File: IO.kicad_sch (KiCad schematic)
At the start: 9 parts, among them J10 Conn_01x04_Pin, J2 Conn_01x02_Pin, J3 Conn_01x02_Pin, J4 Conn_01x02_Pin, J5 Conn_01x02_Pin, J6 Conn_01x02_Pin, J7 Conn_01x04_Pin, J8 Conn_01x04_Pin, J9 Conn_01x04_Pin

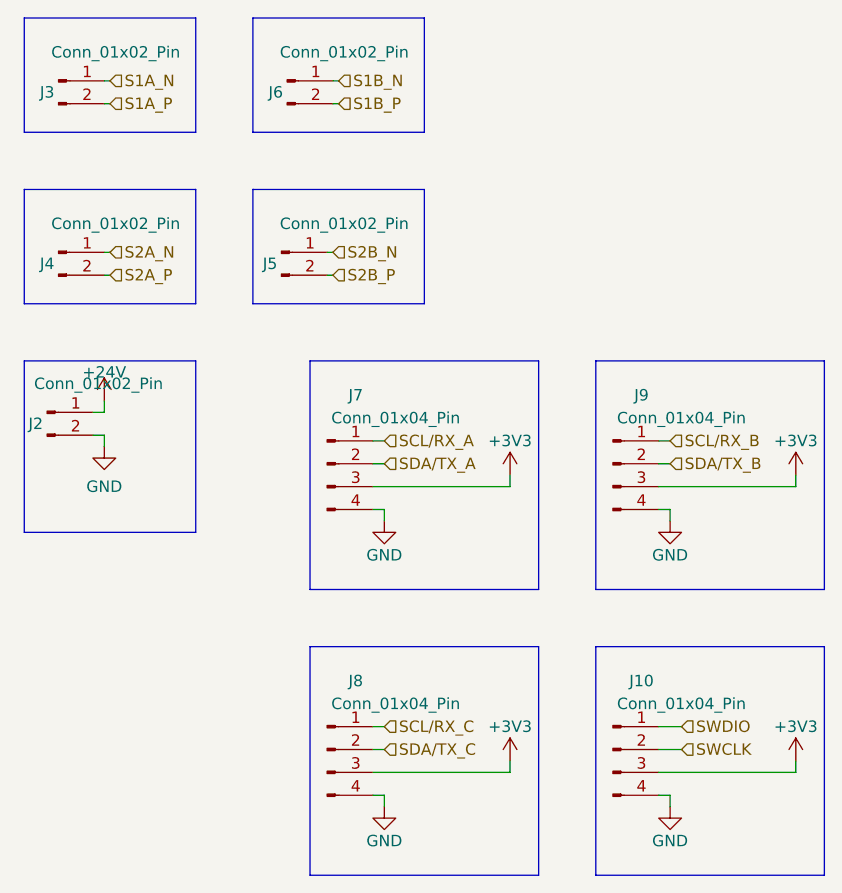
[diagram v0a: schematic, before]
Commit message: added some notes and PDF
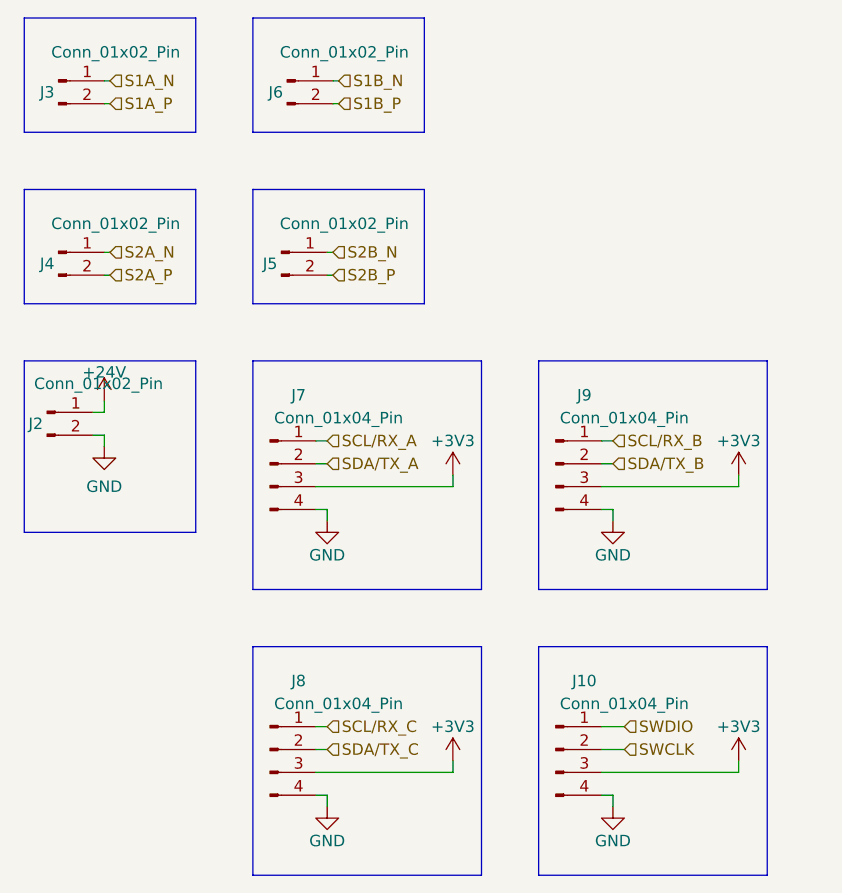
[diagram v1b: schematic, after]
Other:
- moved on the sheet: J10, J7, J8, J9
